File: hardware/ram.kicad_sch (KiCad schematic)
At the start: 17 parts, among them U10 IS42S16320D-6BLI, U4 CCGM1A1

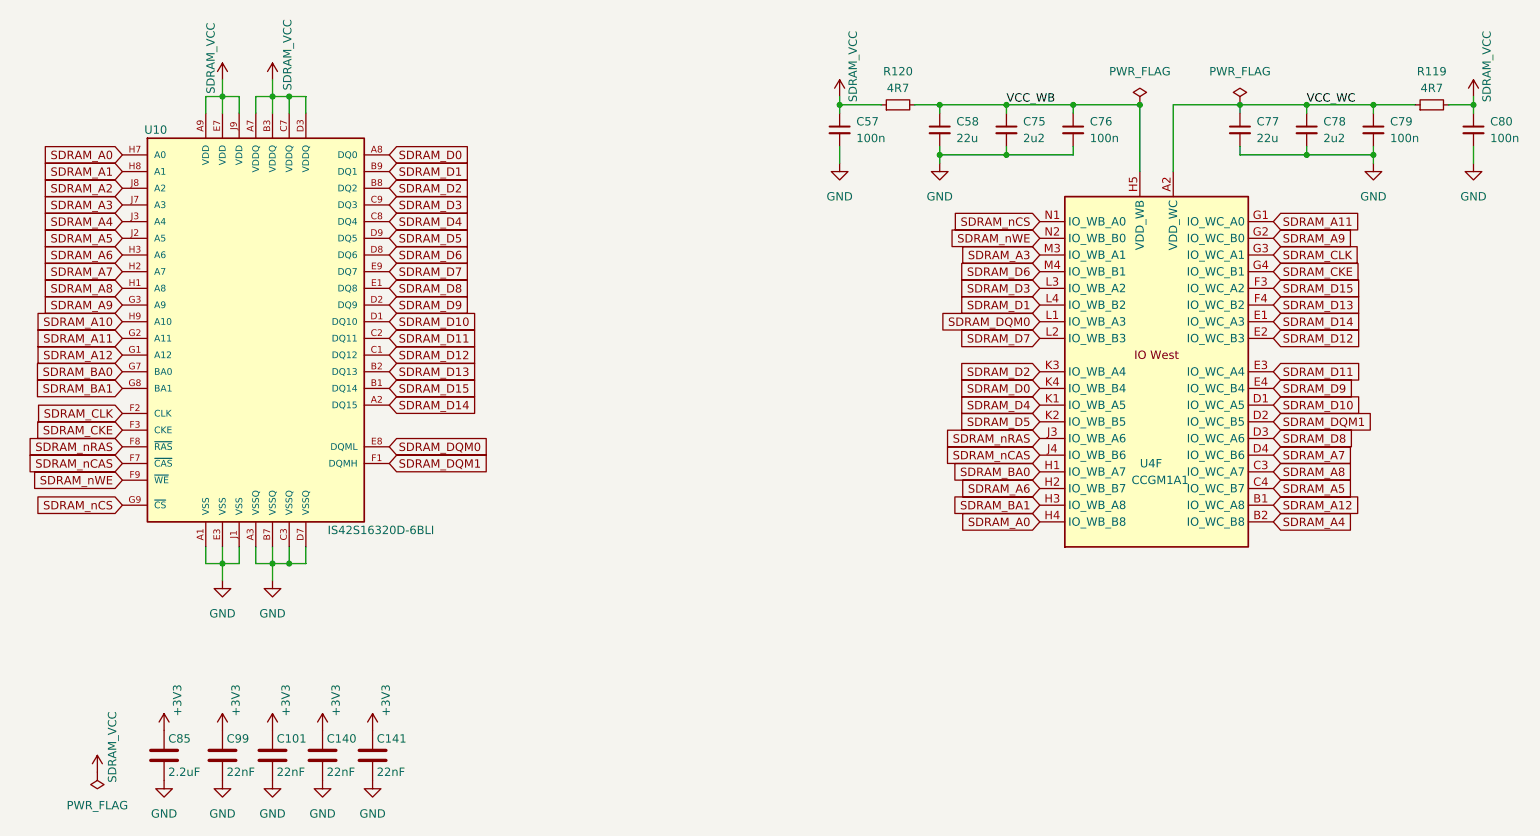
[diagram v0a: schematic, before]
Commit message: Cleanup
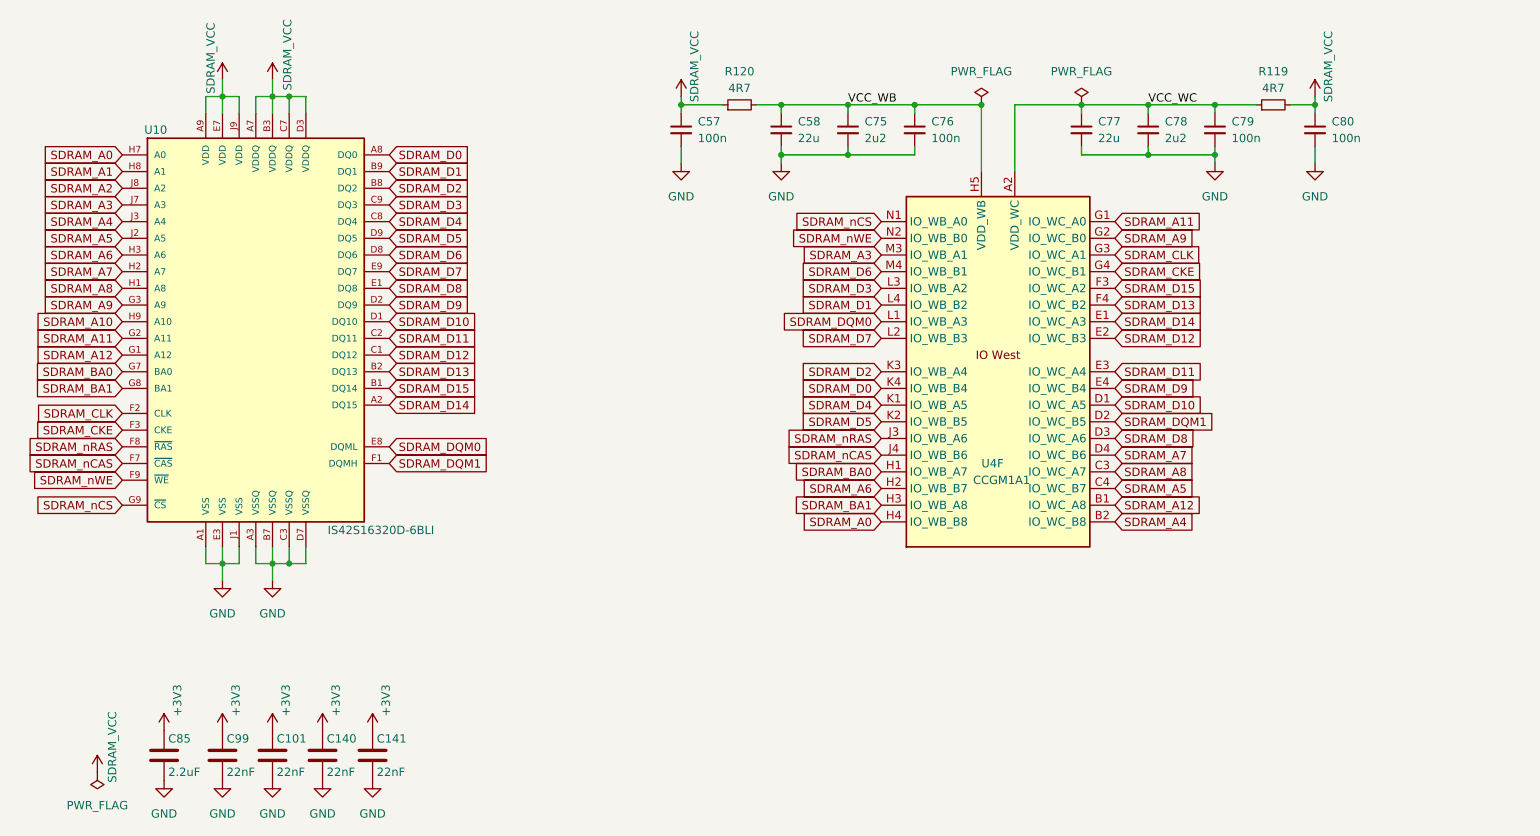
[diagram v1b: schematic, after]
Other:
- moved on the sheet: C57, C58, C75, C76, C77, C78, C79, C80, R119, R120, U4F
